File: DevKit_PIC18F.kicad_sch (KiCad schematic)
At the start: 27 parts, among them J1 PIC_ICSP_ICD, J2 USB_C_Receptacle_USB2.0_16P, J4 RA_PORT, J5 RB_PORT, J6 RD_PORT, J7 RC_PORT, J8 RE_PORT, J9 2P_UART, SW1 SW_DIP, X1 16MHz

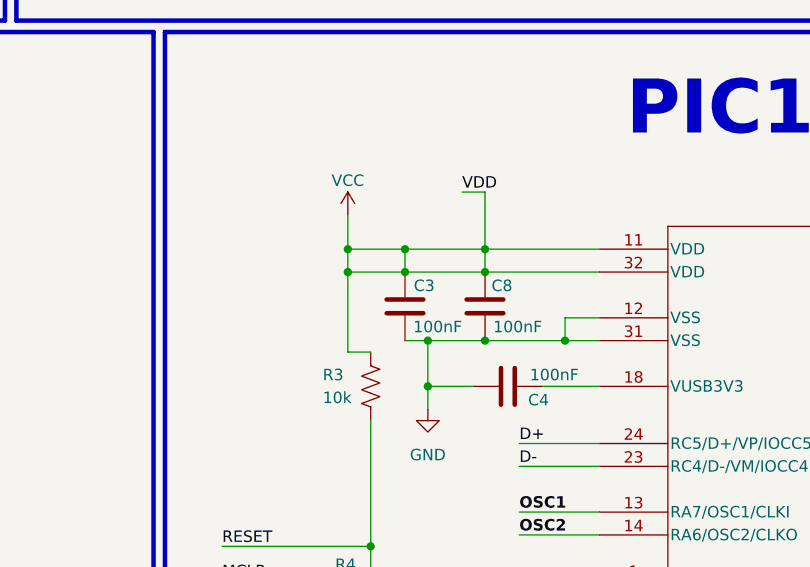
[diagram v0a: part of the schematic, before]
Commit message: refine routing
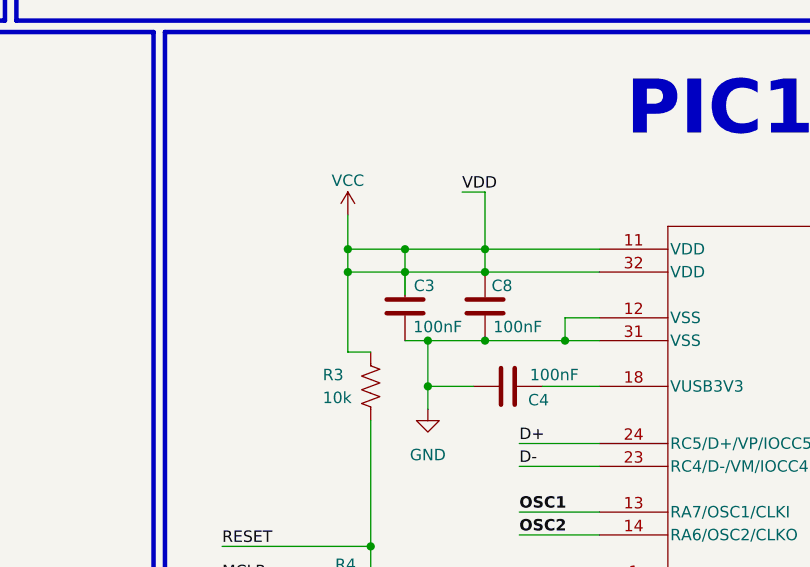
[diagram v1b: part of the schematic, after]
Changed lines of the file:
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@@
+	(wire
+		(pts
+			(xy 114.3 101.6) (xy 114.3 104.14)
+		)
+		(stroke
+			(width 0)
+			(type default)
+		)
+	)
 	(wire
 		(pts
